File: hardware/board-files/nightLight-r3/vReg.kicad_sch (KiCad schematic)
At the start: 14 parts, among them IC1 PAM2401SCADJ, Q1 NMOS, Q2 PMOS

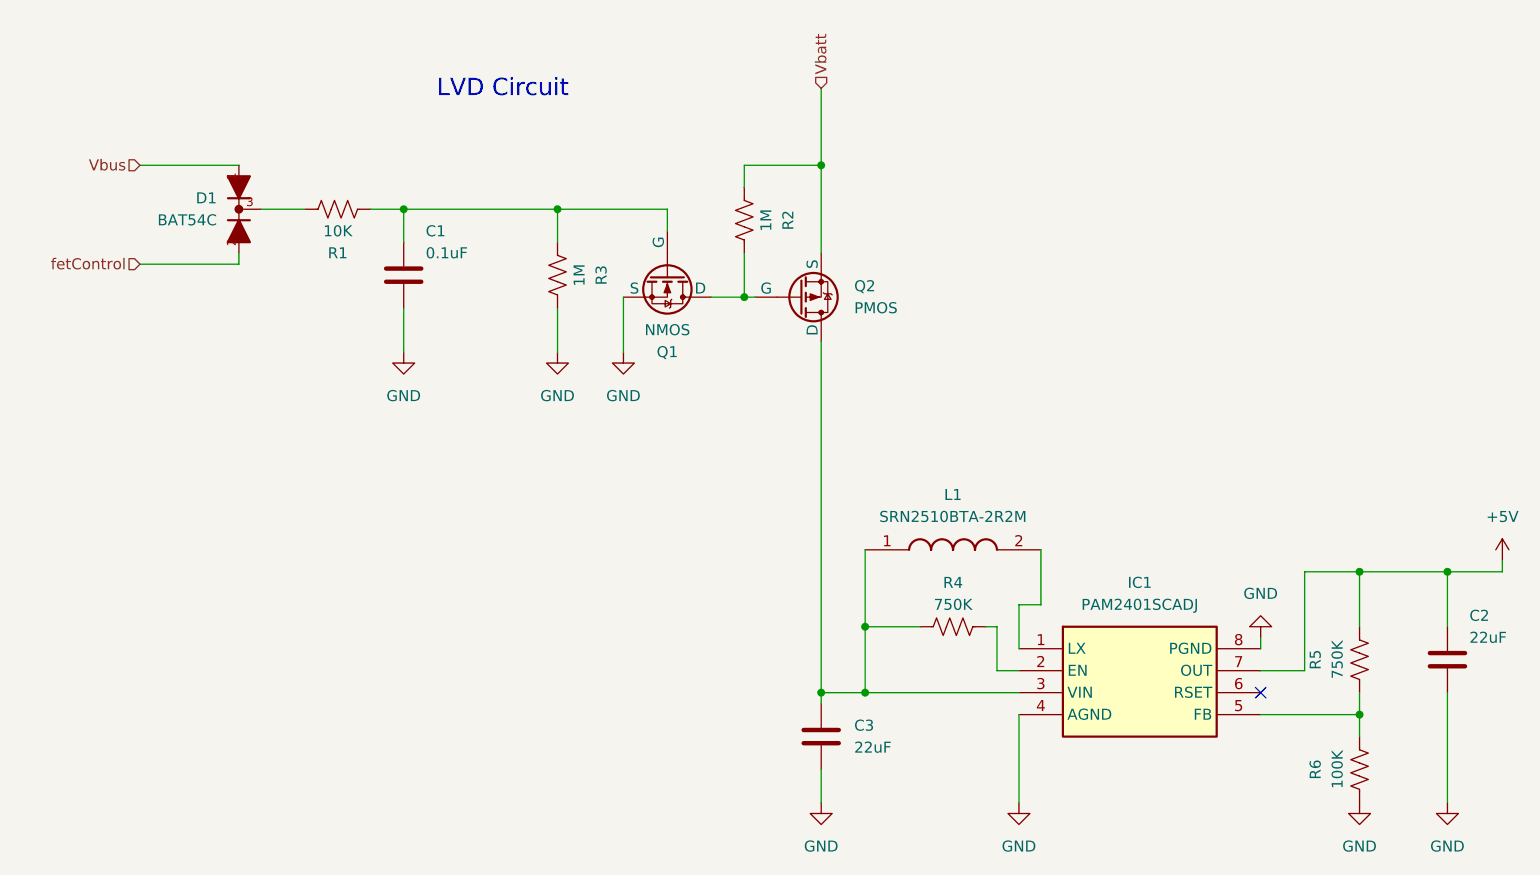
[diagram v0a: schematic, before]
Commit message: PCB rev 3.1 done
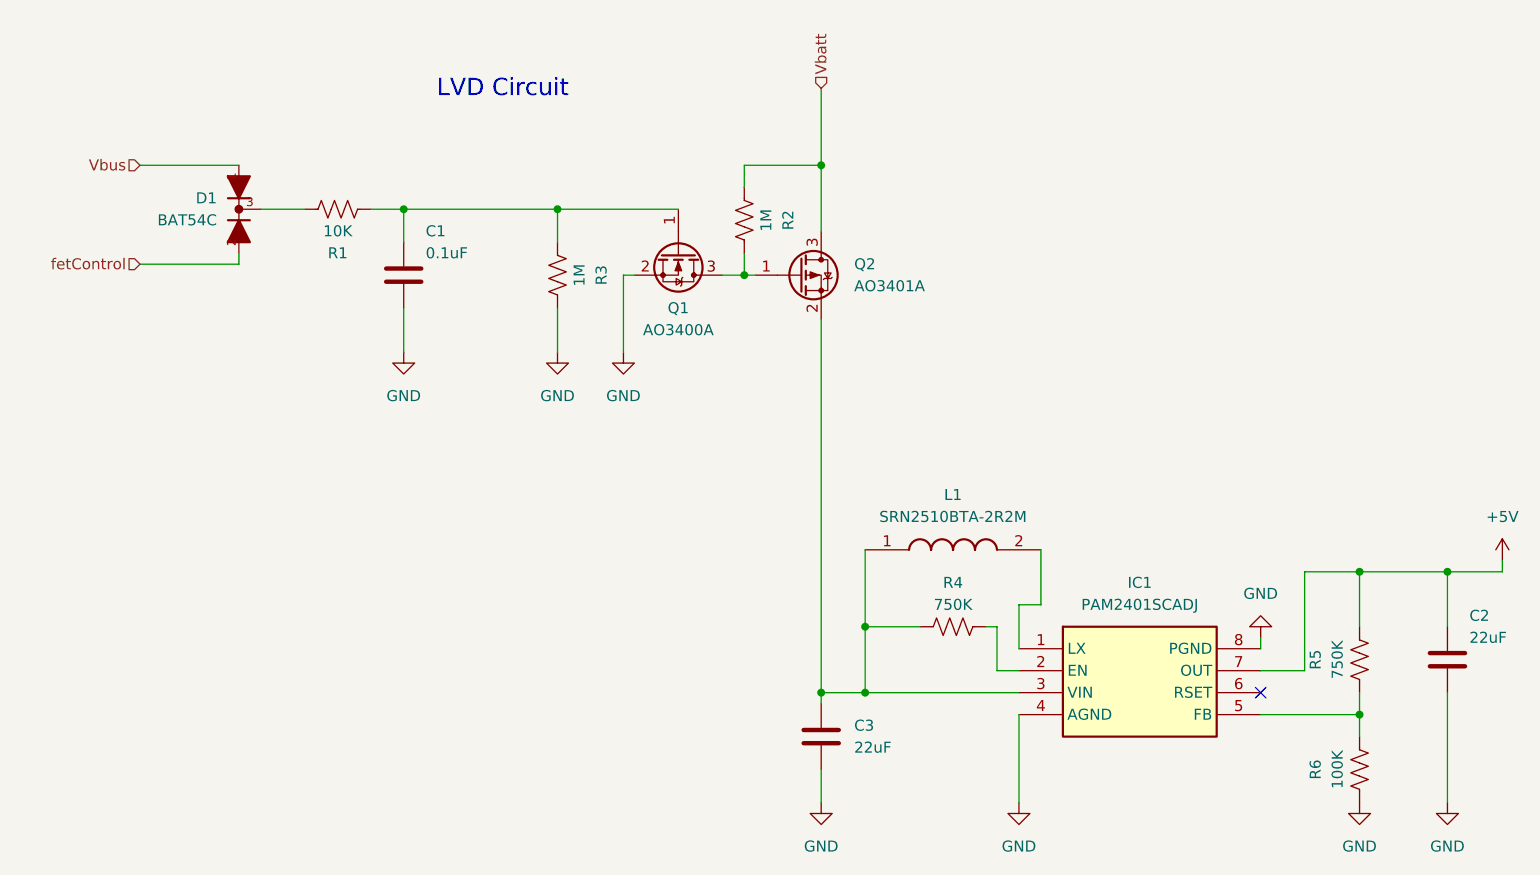
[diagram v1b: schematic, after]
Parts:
- removed Q1: NMOS, IRLML6402TRPBF:SOT95P237X112-3N, symbol Simulation_SPICE:NMOS
- removed Q2: PMOS, IRLML6344TRPBF:SOT95P240X112-3N, symbol Simulation_SPICE:PMOS
- added Q1: AO3400A, Package_TO_SOT_SMD:SOT-23, symbol Transistor_FET:AO3400A
- added Q2: AO3401A, Package_TO_SOT_SMD:SOT-23, symbol Transistor_FET:AO3401A
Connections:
- net GND: now also Q1.2 (S)
- net Vbatt: now also Q2.3 (D)
- net at C3.1, IC1.3 (VIN), L1.1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: now also Q2.2 (S)
- net at C1.1, R1.1, R3.1: now also Q1.1 (G)
- net at R2.2: now also Q1.3 (D), Q2.1 (G)
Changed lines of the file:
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@@
   (junction (at 146.05 66.04) (diameter 0) (color 0 0 0 0)
   )
+  (junction (at 137.16 78.74) (diameter 0) (color 0 0 0 0)
+  )
   (junction (at 146.05 127) (diameter 0) (color 0 0 0 0)
   )
   (junction (at 151.13 119.38) (diameter 0) (color 0 0 0 0)
-  )
-  (junction (at 137.16 81.28) (diameter 0) (color 0 0 0 0)
   )
   (junction (at 151.13 127) (diameter 0) (color 0 0 0 0)
@@
     (stroke (width 0) (type default))
   )
-  (wire (pts (xy 137.16 76.2) (xy 137.16 81.28))
+  (wire (pts (xy 137.16 76.2) (xy 137.16 78.74))
+    (stroke (width 0) (type default))
+  )
+  (wire (pts (xy 134.62 78.74) (xy 137.16 78.74))
     (stroke (width 0) (type default))
   )
@@
     (stroke (width 0) (type default))
   )
-  (wire (pts (xy 115.57 71.12) (xy 128.27 71.12))
-    (stroke (width 0) (type default))
-  )
-  (wire (pts (xy 146.05 66.04) (xy 146.05 76.2))
+  (wire (pts (xy 146.05 66.04) (xy 146.05 73.66))
     (stroke (width 0) (type default))
   )
@@
     (stroke (width 0) (type default))
   )
+  (wire (pts (xy 137.16 78.74) (xy 138.43 78.74))
+    (stroke (width 0) (type default))
+  )
   (wire (pts (xy 218.44 127) (xy 218.44 139.7))
     (stroke (width 0) (type default))
@@
     (stroke (width 0) (type default))
   )
-  (wire (pts (xy 137.16 81.28) (xy 138.43 81.28))
-    (stroke (width 0) (type default))
-  )
   (wire (pts (xy 151.13 119.38) (xy 157.48 119.38))
     (stroke (width 0) (type default))
@@
     (stroke (width 0) (type default))
   )
+  (wire (pts (xy 124.46 78.74) (xy 123.19 78.74))
+    (stroke (width 0) (type default))
+  )
+  (wire (pts (xy 115.57 71.12) (xy 129.54 71.12))
+    (stroke (width 0) (type default))
+  )
   (wire (pts (xy 171.45 116.84) (xy 168.91 116.84))
     (stroke (width 0) (type default))
   )
-  (wire (pts (xy 146.05 86.36) (xy 146.05 127))
+  (wire (pts (xy 146.05 83.82) (xy 146.05 127))
     (stroke (width 0) (type default))
   )
@@
     (stroke (width 0) (type default))
   )
-  (wire (pts (xy 133.35 81.28) (xy 137.16 81.28))
-    (stroke (width 0) (type default))
-  )
   (wire (pts (xy 146.05 57.15) (xy 146.05 66.04))
     (stroke (width 0) (type default))
@@
     (stroke (width 0) (type default))
   )
-  (wire (pts (xy 123.19 81.28) (xy 123.19 87.63))
+  (wire (pts (xy 123.19 78.74) (xy 123.19 87.63))
     (stroke (width 0) (type default))
   )
@@
   )
   (wire (pts (xy 151.13 110.49) (xy 151.13 119.38))
-    (stroke (width 0) (type default))
-  )
-  (wire (pts (xy 128.27 71.12) (xy 128.27 73.66))
     (stroke (width 0) (type default))
   )
@@
         (path "/203033dd-6a13-4262-9a98-8b29445e90e8/e6a767d4-c228-4ec6-8577-23f8c70359e3"
           (reference "R2") (unit 1)
+        )
+      )
+    )
+  )
+  (symbol (lib_id "Transistor_FET:AO3400A") (at 129.54 76.2 270) (unit 1)
+    (in_bom yes) (on_board yes) (dnp no) (fields_autoplaced)
+    (property "Reference" "Q1" (at 129.54 82.55 90)
+      (effects (font (size 1.27 1.27)))
+    )
+    (property "Value" "AO3400A" (at 129.54 85.09 90)
+      (effects (font (size 1.27 1.27)))
+    )
+    (property "Footprint" "Package_TO_SOT_SMD:SOT-23" (at 127.635 81.28 0)
+      (effects (font (size 1.27 1.27) italic) (justify left) hide)
+    )
+    (property "Datasheet" "http://www.aosmd.com/pdfs/datasheet/AO3400A.pdf" (at 125.73 81.28 0)
+      (effects (font (size 1.27 1.27)) (justify left) hide)
+    )
+    (pin "3")
+    (pin "1")
+    (pin "2")
+    (instances
+      (project "nightLight"
+        (path "/203033dd-6a13-4262-9a98-8b29445e90e8/e6a767d4-c228-4ec6-8577-23f8c70359e3"
+          (reference "Q1") (unit 1)
         )
       )
@@
     )
   )
+  (symbol (lib_id "Transistor_FET:AO3401A") (at 143.51 78.74 0) (unit 1)
+    (in_bom yes) (on_board yes) (dnp no) (fields_autoplaced)
+    (property "Reference" "Q2" (at 149.86 77.47 0)
+      (effects (font (size 1.27 1.27)) (justify left))
+    )
+    (property "Value" "AO3401A" (at 149.86 80.01 0)
+      (effects (font (size 1.27 1.27)) (justify left))
+    )
+    (property "Footprint" "Package_TO_SOT_SMD:SOT-23" (at 148.59 80.645 0)
+      (effects (font (size 1.27 1.27) italic) (justify left) hide)
+    )
+    (property "Datasheet" "http://www.aosmd.com/pdfs/datasheet/AO3401A.pdf" (at 148.59 82.55 0)
+      (effects (font (size 1.27 1.27)) (justify left) hide)
+    )
+    (pin "3")
+    (pin "2")
+    (pin "1")
+    (instances
+      (project "nightLight"
+        (path "/203033dd-6a13-4262-9a98-8b29445e90e8/e6a767d4-c228-4ec6-8577-23f8c70359e3"
+          (reference "Q2") (unit 1)
+        )
+      )
+    )
+  )
   (symbol (lib_id "power:GND") (at 123.19 87.63 0) (unit 1)
     (in_bom yes) (on_board yes) (dnp no) (fields_autoplaced)
@@
         (path "/203033dd-6a13-4262-9a98-8b29445e90e8/e6a767d4-c228-4ec6-8577-23f8c70359e3"
           (reference "#PWR03") (unit 1)
-        )
-      )
-    )
-  )
-  (symbol (lib_id "Simulation_SPICE:NMOS") (at 128.27 78.74 270) (unit 1)
-    (in_bom yes) (on_board yes) (dnp no)
-    (property "Reference" "Q1" (at 128.27 87.63 90)
-      (effects (font (size 1.27 1.27)))
-    )
-    (property "Value" "NMOS" (at 128.27 85.09 90)
-      (effects (font (size 1.27 1.27)))
-    )
-    (property "Footprint" "IRLML6402TRPBF:SOT95P237X112-3N" (at 130.81 83.82 0)
-      (effects (font (size 1.27 1.27)) hide)
-    )
-    (property "Datasheet" "https://ngspice.sourceforge.io/docs/ngspice-html-manual/manual.xhtml#cha_MOSFETs" (at 115.57 78.74 0)
-      (effects (font (size 1.27 1.27)) hide)
-    )
-    (property "Sim.Device" "NMOS" (at 111.125 78.74 0)
-      (effects (font (size 1.27 1.27)) hide)
-    )
-    (property "Sim.Type" "VDMOS" (at 109.22 78.74 0)
-      (effects (font (size 1.27 1.27)) hide)
-    )
-    (property "Sim.Pins" "1=D 2=G 3=S" (at 113.03 78.74 0)
-      (effects (font (size 1.27 1.27)) hide)
-    )
-    (pin "1")
-    (pin "2")
-    (pin "3")
-    (instances
-      (project "nightLight"
-        (path "/203033dd-6a13-4262-9a98-8b29445e90e8/e6a767d4-c228-4ec6-8577-23f8c70359e3"
-          (reference "Q1") (unit 1)
         )
       )
@@
         )
       )
-    )
-  )
-  (symbol (lib_id "Simulation_SPICE:PMOS") (at 143.51 81.28 0) (mirror x) (unit 1)
-    (in_bom yes) (on_board yes) (dnp no)
-    (property "Reference" "Q2" (at 149.86 80.01 0)
-      (effects (font (size 1.27 1.27)) (justify left))
-    )
-    (property "Value" "PMOS" (at 149.86 82.55 0)
-      (effects (font (size 1.27 1.27)) (justify left))
-    )
-    (property "Footprint" "IRLML6344TRPBF:SOT95P240X112-3N" (at 148.59 83.82 0)
-      (effects (font (size 1.27 1.27)) hide)
-    )
-    (property "Datasheet" "https://ngspice.sourceforge.io/docs/ngspice-html-manual/manual.xhtml#cha_MOSFETs" (at 143.51 68.58 0)
-      (effects (font (size 1.27 1.27)) hide)
-    )
-    (property "Sim.Device" "PMOS" (at 143.51 64.135 0)
-      (effects (font (size 1.27 1.27)) hide)
-    )
-    (property "Sim.Type" "VDMOS" (at 143.51 62.23 0)
-      (effects (font (size 1.27 1.27)) hide)
-    )
-    (property "Sim.Pins" "1=D 2=G 3=S" (at 143.51 66.04 0)
-      (effects (font (size 1.27 1.27)) hide)
-    )
-    (pin "2")
-    (pin "3")
-    (pin "1")
-    (instances
-      (project "nightLight"
-        (path "/203033dd-6a13-4262-9a98-8b29445e90e8/e6a767d4-c228-4ec6-8577-23f8c70359e3"
-          (reference "Q2") (unit 1)
-        )
-      )
